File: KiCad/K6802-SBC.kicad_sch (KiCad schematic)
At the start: 47 parts, among them J1 Barrel_Jack_Switch, J2 SBC6303 BUS, J3 SERIAL JP, SW1 POWER, SW2 RESET, U1 74LS00, U2 74LS00, U3 MC6802, U4 74LS138, U5 HM628128D_DIP32_SOP32, U6 74HC4060, U7 27C256, U8 MC6850, Y1 4MHz, Y2 19.6608MHz

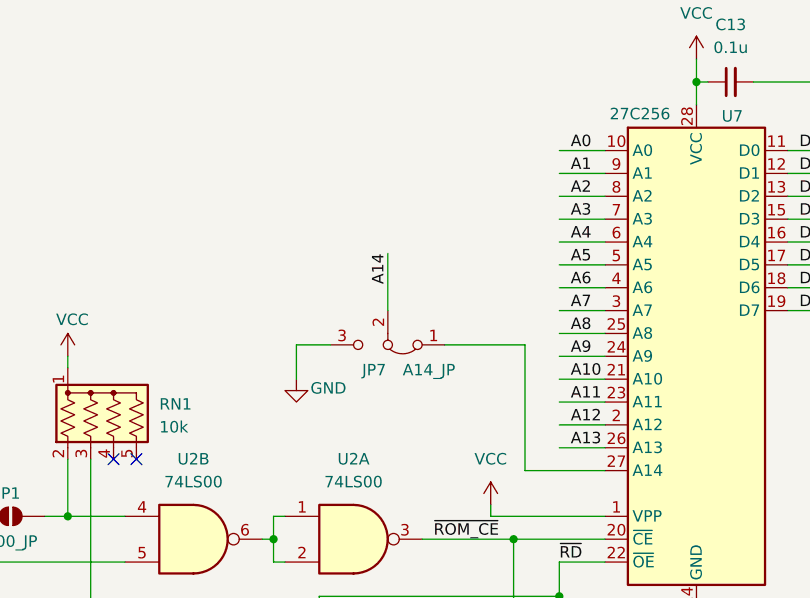
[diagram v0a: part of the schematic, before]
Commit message: プリントパターン作成、ガーバーデータ出力
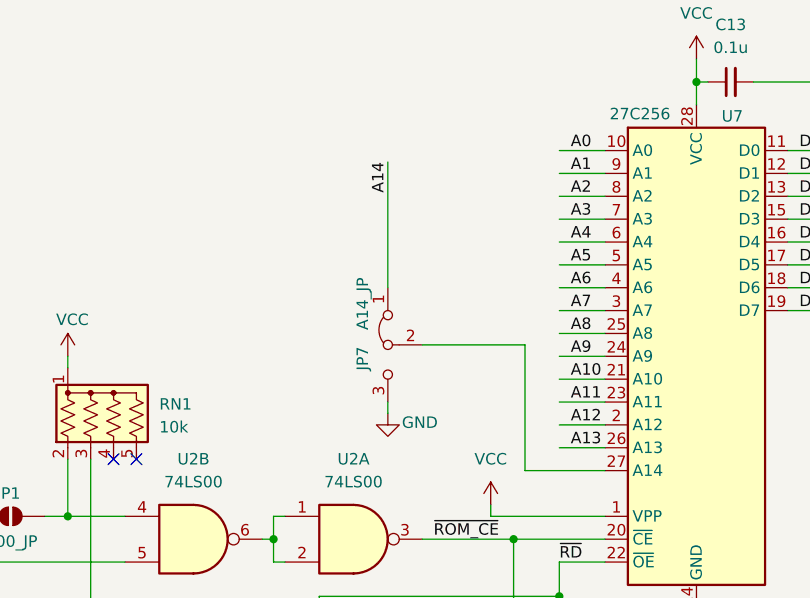
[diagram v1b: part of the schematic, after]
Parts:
- C1, C10, C11, C12, C13, C14, C2, C4, C6, C7, C8, C9: footprint (none) -> Capacitor_THT:C_Disc_D3.0mm_W2.0mm_P2.50mm
- C3, C5: footprint (none) -> Capacitor_THT:CP_Radial_D5.0mm_P2.50mm
- D1: footprint (none) -> Diode_THT:D_A-405_P10.16mm_Horizontal
- D2: footprint (none) -> LED_THT:LED_D3.0mm
- J1: footprint (none) -> Connector_BarrelJack:BarrelJack_Horizontal
- J3: footprint (none) -> Connector_PinHeader_2.54mm:PinHeader_1x06_P2.54mm_Horizontal
- JP1, JP2, JP3, JP4, JP5: footprint (none) -> Jumper:SolderJumper-2_P1.3mm_Open_RoundedPad1.0x1.5mm
- JP6: footprint (none) -> Jumper:SolderJumper-2_P1.3mm_Bridged_RoundedPad1.0x1.5mm
- JP7, SW1: footprint (none) -> Connector_PinHeader_2.54mm:PinHeader_1x03_P2.54mm_Vertical
- R1, R3, R4: footprint (none) -> Resistor_THT:R_Axial_DIN0207_L6.3mm_D2.5mm_P10.16mm_Horizontal
- SW2: footprint (none) -> Button_Switch_THT:SW_PUSH_6mm
- U1, U2: footprint (none) -> Package_DIP:DIP-14_W7.62mm_Socket
- U3: footprint Package_DIP:DIP-40_W15.24mm -> Package_DIP:DIP-40_W15.24mm_Socket
- U4, U6: footprint (none) -> Package_DIP:DIP-16_W7.62mm_Socket
- U5: footprint (none) -> Package_DIP:DIP-32_W15.24mm_Socket
- U7: footprint Package_DIP:DIP-28_W15.24mm -> Package_DIP:DIP-28_W15.24mm_Socket
- U8: footprint Package_DIP:DIP-24_W15.24mm -> Package_DIP:DIP-24_W15.24mm_Socket
- Y1, Y2: footprint (none) -> Crystal:Crystal_HC49-U_Vertical
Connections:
- net A14: now also JP7.1 (A); no longer JP7.2 (C)
- net at U7.27 (A14): now also JP7.2 (C); no longer JP7.1 (A)
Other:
- moved on the sheet: JP7
